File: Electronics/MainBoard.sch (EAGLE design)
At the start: 11 parts, among them J1 1X2-3.5MM

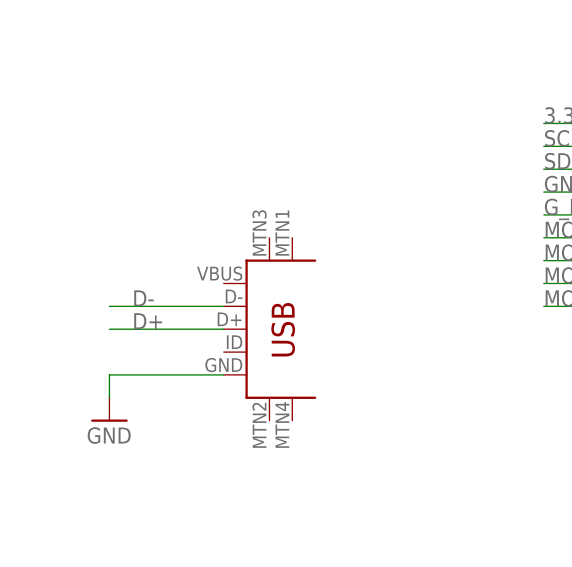
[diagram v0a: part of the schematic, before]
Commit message: mbed code
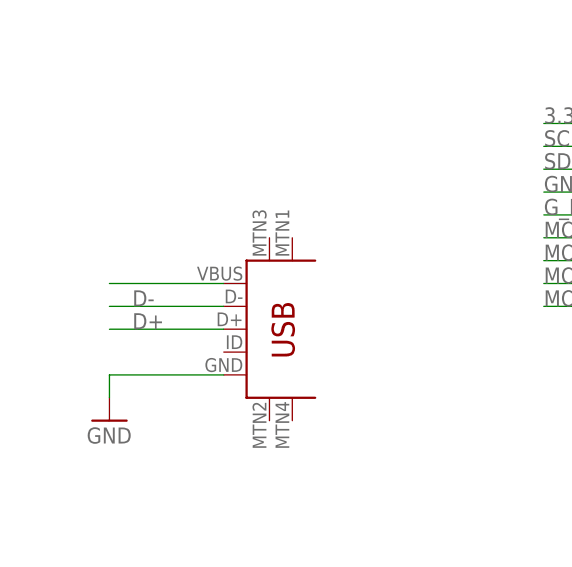
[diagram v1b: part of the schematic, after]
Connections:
- new net N$1: U$1.VBUS
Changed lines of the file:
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@@
+</segment>
+</net>
+<net name="N$1" class="0">
+<segment>
+<pinref part="U$1" gate="G$1" pin="VBUS"/>
+<wire x1="-17.78" y1="147.32" x2="-30.48" y2="147.32" width="0.1524" layer="91"/>
 </segment>
 </net>

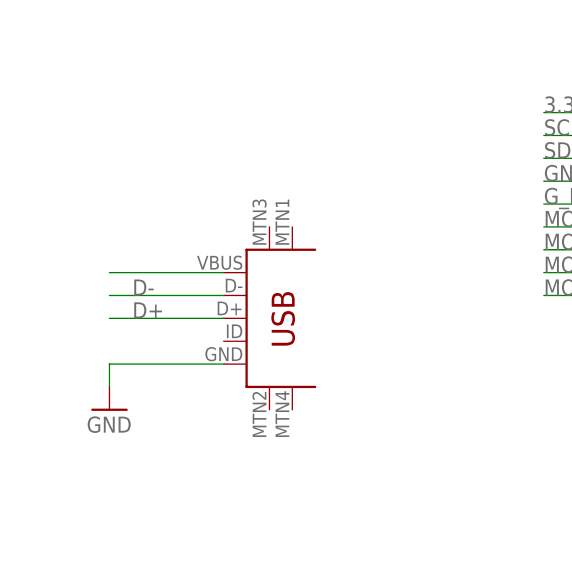
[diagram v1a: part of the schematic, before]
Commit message: main board edits
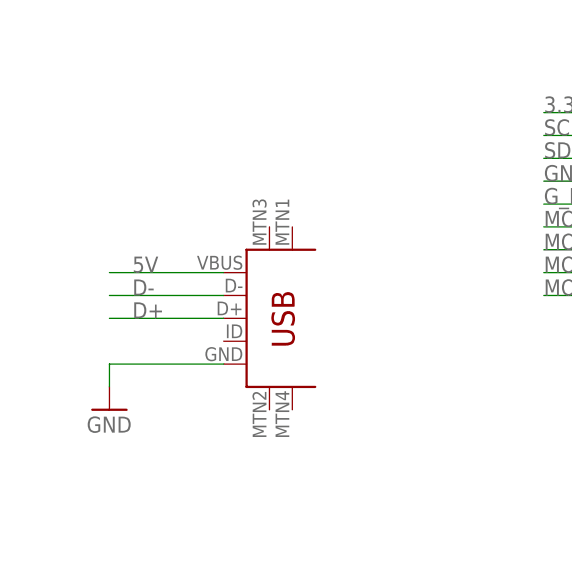
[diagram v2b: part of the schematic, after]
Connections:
- removed net N$1: U$1.VBUS
- net 5V: now also U$1.VBUS
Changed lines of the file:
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@@
 <label x="53.34" y="104.14" size="1.778" layer="95"/>
+</segment>
+<segment>
+<pinref part="U$1" gate="G$1" pin="VBUS"/>
+<wire x1="-17.78" y1="147.32" x2="-30.48" y2="147.32" width="0.1524" layer="91"/>
+<label x="-27.94" y="147.32" size="1.778" layer="95"/>
 </segment>
 </net>
@@
 <segment>
 <pinref part="U$1" gate="G$1" pin="D+"/>
-<wire x1="-17.78" y1="142.24" x2="-30.48" y2="142.24" width="0.1524" layer="91"/>
+<wire x1="-17.78" y1="142.24" x2="-22.86" y2="142.24" width="0.1524" layer="91"/>
 <label x="-27.94" y="142.24" size="1.778" layer="95"/>
+<wire x1="-22.86" y1="142.24" x2="-30.48" y2="142.24" width="0.1524" layer="91"/>
 </segment>
 </net>
@@
 <segment>
 <pinref part="U$1" gate="G$1" pin="D-"/>
-<wire x1="-17.78" y1="144.78" x2="-30.48" y2="144.78" width="0.1524" layer="91"/>
+<wire x1="-17.78" y1="144.78" x2="-27.94" y2="144.78" width="0.1524" layer="91"/>
 <label x="-27.94" y="144.78" size="1.778" layer="95"/>
-</segment>
-</net>
-<net name="N$1" class="0">
-<segment>
-<pinref part="U$1" gate="G$1" pin="VBUS"/>
-<wire x1="-17.78" y1="147.32" x2="-30.48" y2="147.32" width="0.1524" layer="91"/>
-</segment>
-</net>
+<wire x1="-27.94" y1="144.78" x2="-30.48" y2="144.78" width="0.1524" layer="91"/>
+</segment>
+</net>

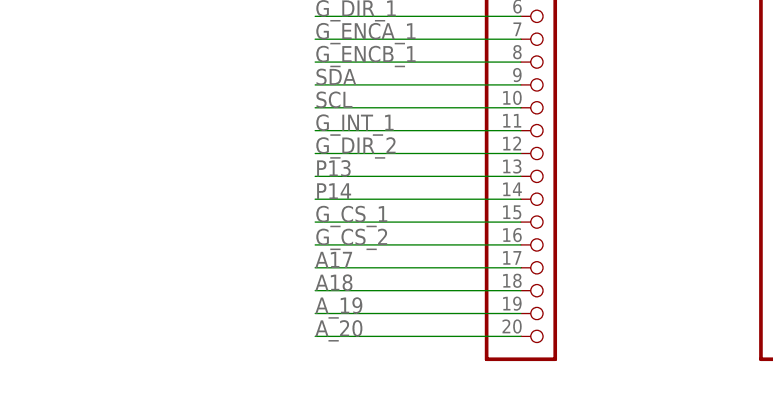
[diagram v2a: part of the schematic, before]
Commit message: board updates
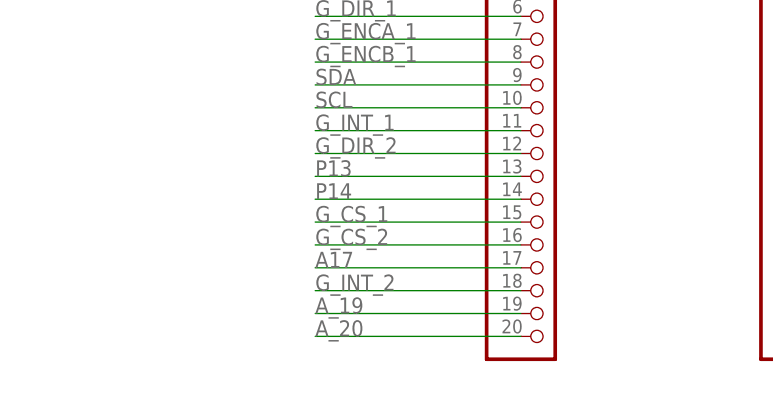
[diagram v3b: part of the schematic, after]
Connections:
- removed net A18: JP1.18
- net G_INT_2: now also JP1.18
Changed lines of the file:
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@@
-</segment>
-</net>
-<net name="A18" class="0">
-<segment>
-<pinref part="JP1" gate="A" pin="18"/>
-<wire x1="15.24" y1="63.5" x2="-7.62" y2="63.5" width="0.1524" layer="91"/>
-<label x="-7.62" y="63.5" size="1.778" layer="95"/>
 </segment>
 </net>
@@
 <label x="17.78" y="154.94" size="1.778" layer="95"/>
 </segment>
-</net>
+<segment>
+<pinref part="JP1" gate="A" pin="18"/>
+<wire x1="15.24" y1="63.5" x2="-7.62" y2="63.5" width="0.1524" layer="91"/>
+<label x="-7.62" y="63.5" size="1.778" layer="95"/>
+</segment>
+</net>
